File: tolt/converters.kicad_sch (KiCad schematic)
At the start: 45 parts, among them J11 Conn_01x05, U14 AMS1117-3.3, U15 LP5907MFX-3.3, U16 TPS62173DSG, U24 LTC7138xMSE

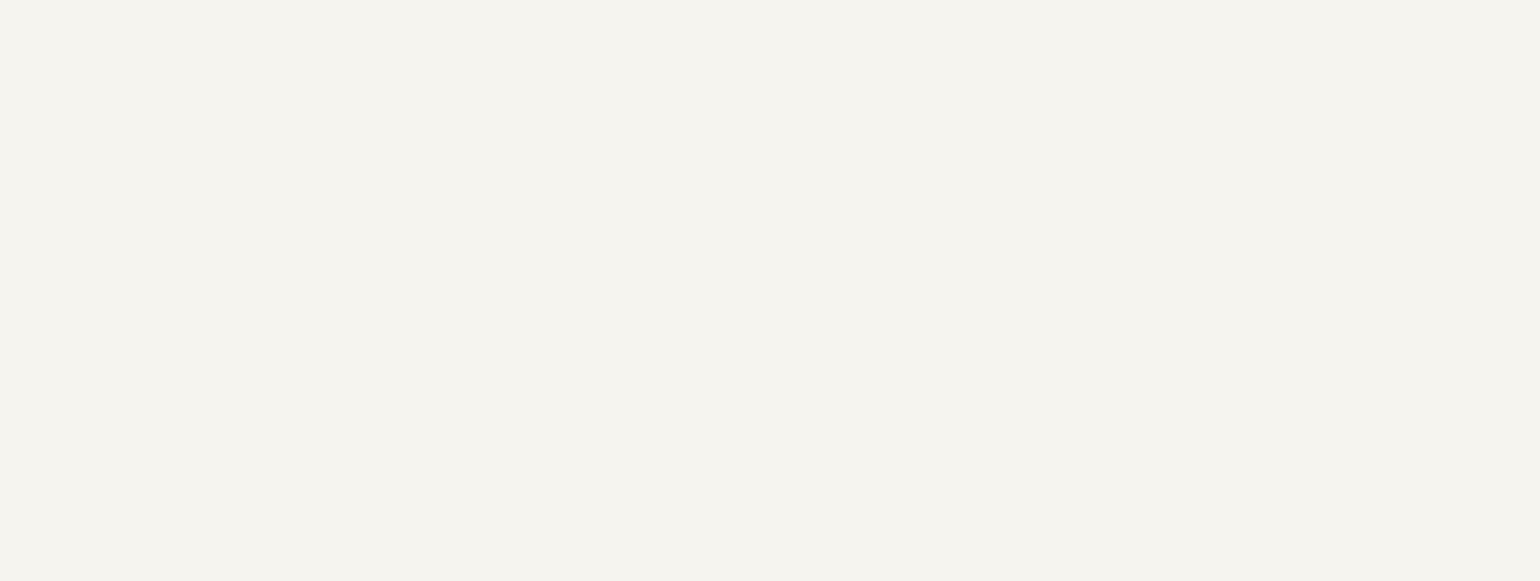
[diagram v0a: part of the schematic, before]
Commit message: 12v
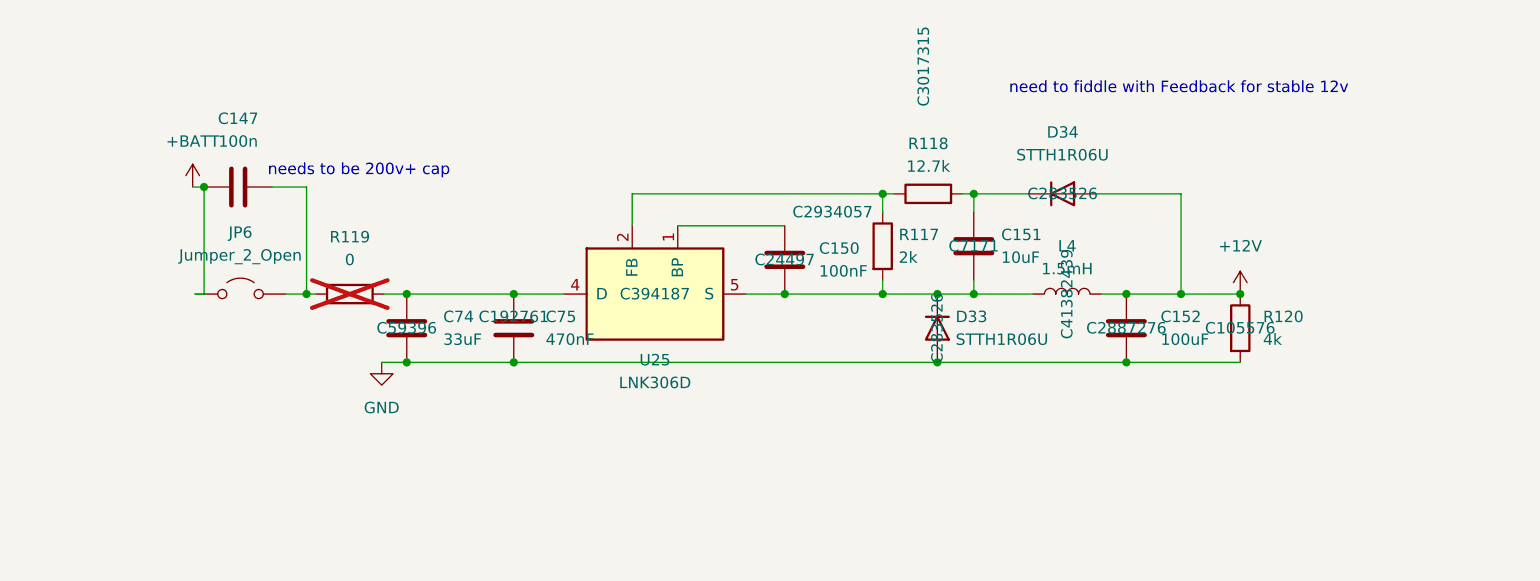
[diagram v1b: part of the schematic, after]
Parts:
- added C147: 100n, Capacitor_SMD:C_1210_3225Metric, symbol Device:C
- added C150: 100nF, Capacitor_SMD:C_1206_3216Metric_Pad1.33x1.80mm_HandSolder, symbol Device:C
- added C151: 10uF, Capacitor_Tantalum_SMD:CP_EIA-3216-18_Kemet-A, symbol Device:C
- added C152: 100uF, Capacitor_SMD:CP_Elec_6.3x5.4, symbol Device:C
- added C74: 33uF, Capacitor_THT:CP_Radial_D10.0mm_P2.50mm_P5.00mm, symbol Device:C
- added C75: 470nF, Capacitor_SMD:C_1210_3225Metric, symbol Device:C
- added D33, D34: STTH1R06U, Diode_SMD:D_SMB, symbol Device:D
- added JP6: Jumper_2_Open, Connector_PinHeader_2.54mm:PinHeader_1x02_P2.54mm_Vertical, symbol Jumper:Jumper_2_Open
- added L4: 1.5mH, Inductor_SMD:L_Bourns_SRN8040TA, symbol Device:L
- added R117: 2k, Resistor_SMD:R_2512_6332Metric, symbol Device:R
- added R118: 12.7k, Resistor_SMD:R_1206_3216Metric, symbol Device:R
- added R119: 0, Resistor_SMD:R_0603_1608Metric, symbol Device:R
- added R120: 4k, Resistor_SMD:R_0603_1608Metric, symbol Device:R
- added U25: LNK306D, EasyEDA2KiCad:SO-8C_7P-L4.9-W3.9-P1.27-LS6.0-BL-PE3, symbol Regulator_Switching:LNK306D
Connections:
- net +12V: now also C152.1, D34.2 (A), L4.2, R120.1
- net +BATT: now also C147.1, JP6.1 (A)
- net GND: now also C152.2, C74.2, C75.2, D33.2 (A), R120.2
- new net: R117.1, R118.1, U25.2 (FB)
- new net: C151.1, D34.1 (K), R118.2
- new net: C147.2, JP6.2 (B), R119.1
- new net: C74.1, C75.1, R119.2, U25.4 (D)
- new net: C150.2, C151.2, D33.1 (K), L4.1, R117.2, U25.5 (S), U25.6 (S), U25.7 (S), U25.8 (S)
- new net: C150.1, U25.1 (BP)
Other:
- note added: "need to fiddle with Feedback for stable 12v"
- note added: "needs to be 200v+ cap"
